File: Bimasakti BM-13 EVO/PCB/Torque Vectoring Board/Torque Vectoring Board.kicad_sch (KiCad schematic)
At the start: 34 parts, among them J1 SIGNAL 1, J2 SIGNAL 2, J3 wsout1, J4 wsout2, U3 SN65HVD230, U4 SN65HVD230, U5 ADS1115IDGS

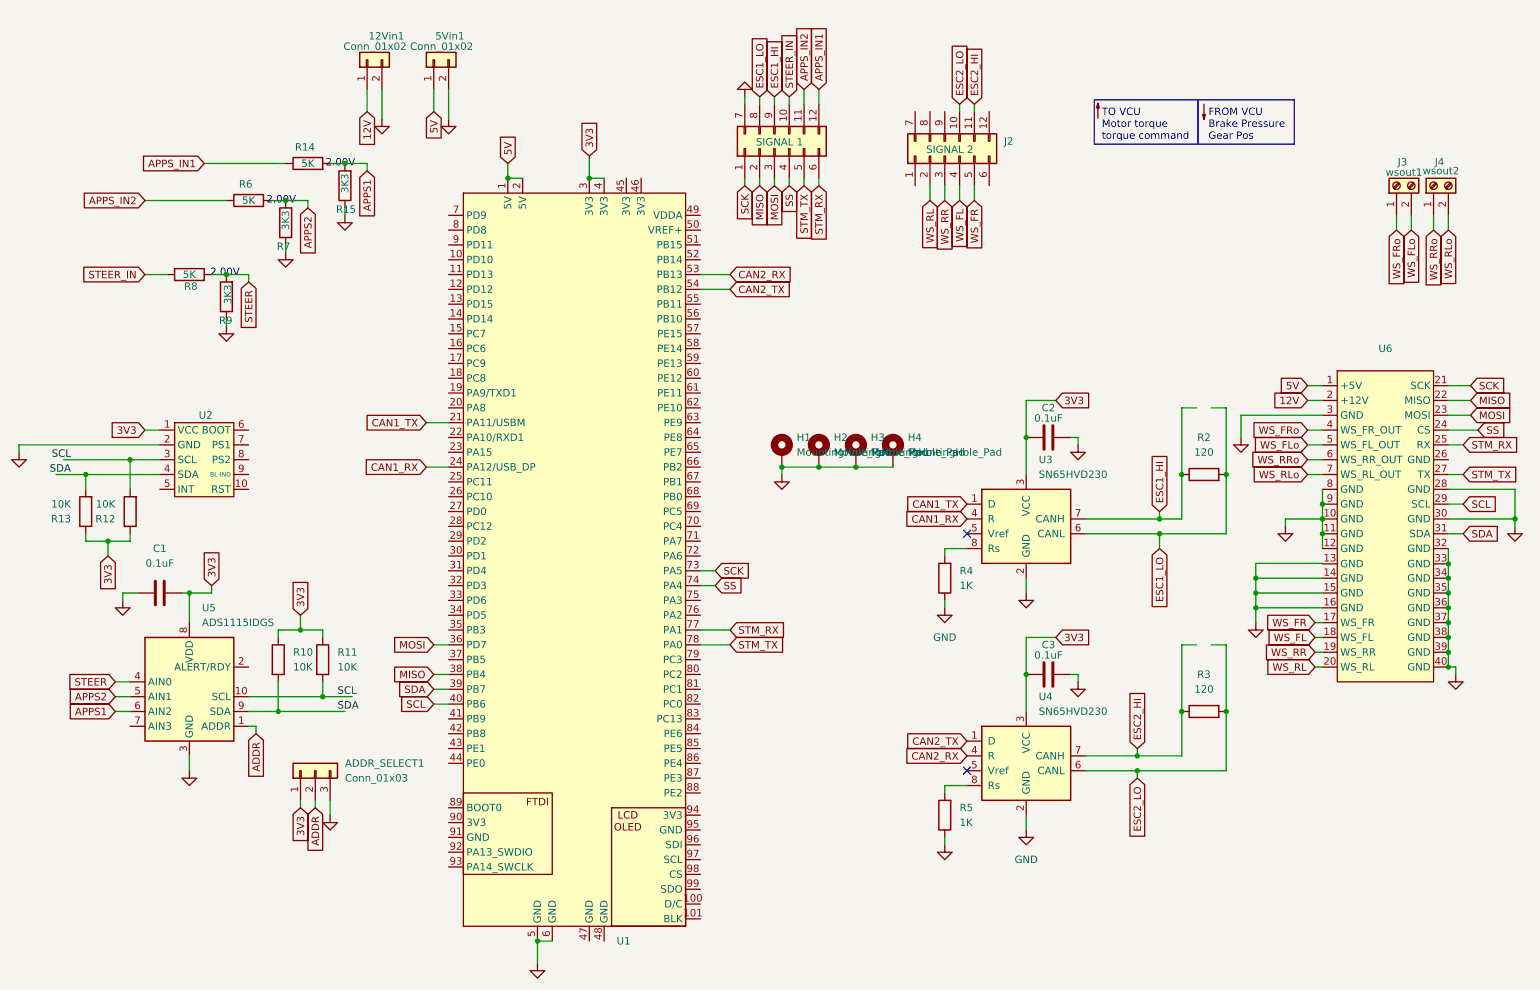
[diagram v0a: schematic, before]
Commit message: pdm and tv fix
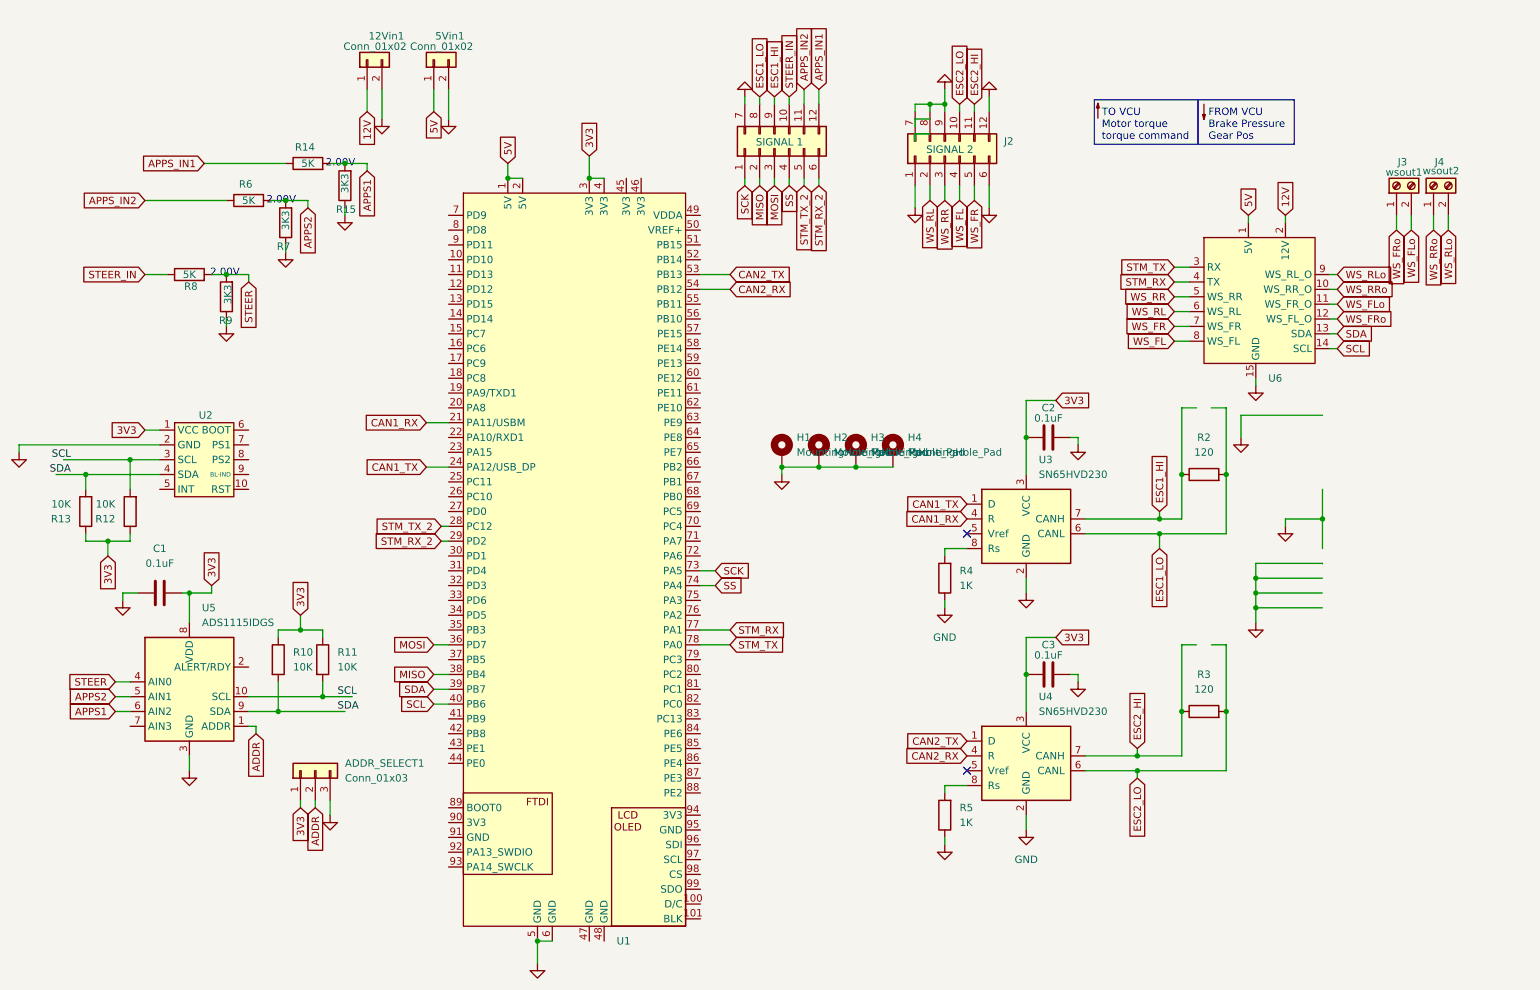
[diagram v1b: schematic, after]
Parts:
- removed U6: ~, 0_CUSTOM_PCB:wheelspeed, symbol 0_CUSTOM_PCB:Wheelspeed
- added U6: ~, 0_WHEELSPEED:Untitled, symbol 0_wheelspeed:wheelspeed
- J3, J4: footprint TerminalBlock_Phoenix:TerminalBlock_Phoenix_PT-1,5-2-5.0-H_1x02_P5.00mm_Horizontal -> Connector_Molex:Molex_Nano-Fit_105309-xx02_1x02_P2.50mm_Vertical
- R10, R11, R12, R13, R14, R15, R2, R3, R4, R5, R6, R7, R8, R9: footprint Resistor_SMD:R_0805_2012Metric -> Resistor_SMD:R_0603_1608Metric
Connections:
- net 12V: now also U6.2 (12V)
- net 5V: now also U6.1 (5V)
- net CAN1_RX: now also U1.21 (PA11/USBM); no longer U1.24 (PA12/USB_DP)
- net CAN1_TX: now also U1.24 (PA12/USB_DP); no longer U1.21 (PA11/USBM)
- net CAN2_RX: now also U1.54 (PB12); no longer U1.53 (PB13)
- net CAN2_TX: now also U1.53 (PB13); no longer U1.54 (PB12)
- net GND: now also J2.1 (Pin_1), J2.12 (Pin_12), J2.6 (Pin_6), J2.7 (Pin_7), J2.8 (Pin_8), J2.9 (Pin_9), U6.15 (GND)
- net SCL: now also U6.14 (SCL)
- net SDA: now also U6.13 (SDA)
- net STM_RX: now also U6.4 (TX); no longer J1.6 (Pin_6)
- net STM_TX: now also U6.3 (RX); no longer J1.5 (Pin_5)
- net WS_FL: now also U6.8 (WS_FL)
- net WS_FLo: now also U6.11 (WS_FR_O)
- net WS_FR: now also U6.7 (WS_FR)
- net WS_FRo: now also U6.12 (WS_FL_O)
- net WS_RL: now also U6.6 (WS_RL)
- net WS_RLo: now also U6.9 (WS_RL_O)
- net WS_RR: now also U6.5 (WS_RR)
- net WS_RRo: now also U6.10 (WS_RR_O)
- net STM_TX_2: now reaches U1.28 (PC12)
- net STM_TX_2: now also J1.5 (Pin_5)
- net STM_RX_2: now reaches U1.29 (PD2)
- net STM_RX_2: now also J1.6 (Pin_6)
